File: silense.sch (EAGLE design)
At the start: 222 parts, among them IC1 AD8334ACPZ, IC3 LT8471EFE#PBF, J1 FMC-LPC

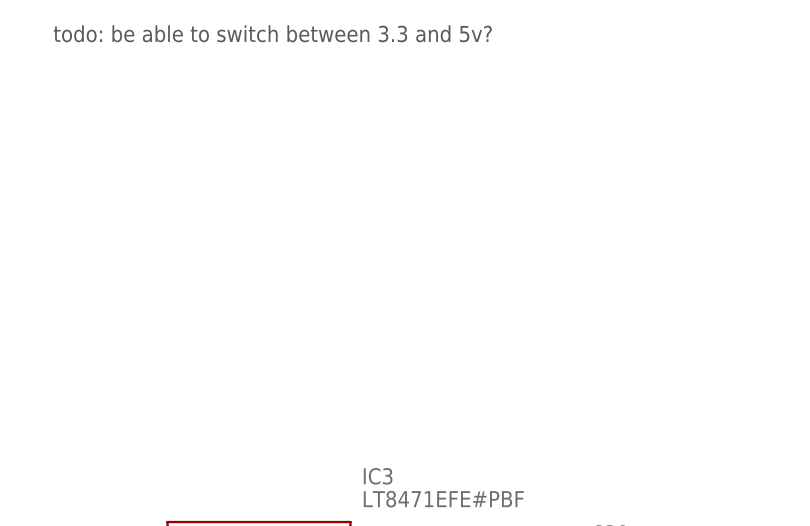
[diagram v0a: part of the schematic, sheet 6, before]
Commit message: added todos
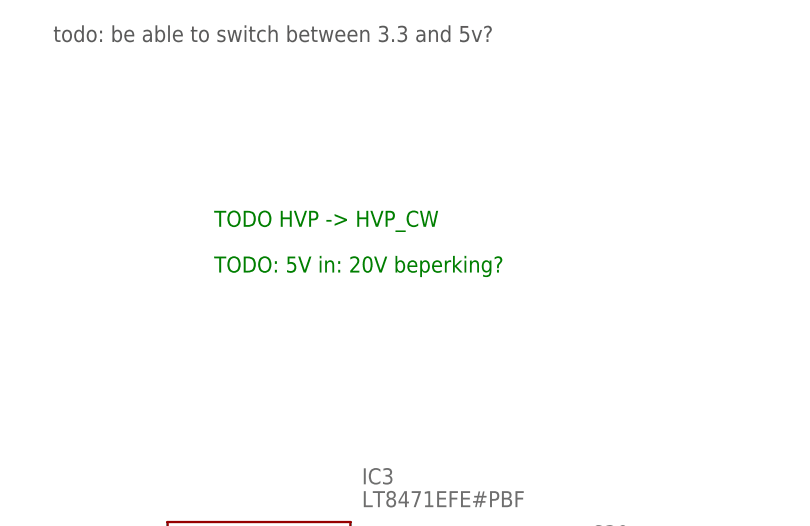
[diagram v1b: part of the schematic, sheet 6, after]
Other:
- note added: "TODO HVP -> HVP_CW"
- note added: "TODO: 5V in: 20V beperking?"
- note added: "TODO: Power supplies"
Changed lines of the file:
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@@
 <?xml version="1.0" encoding="utf-8"?>
 <!DOCTYPE eagle SYSTEM "eagle.dtd">
-<eagle version="9.5.1">
+<eagle version="9.5.0">
 <drawing>
 <settings>
@@
 <setting verticaltext="up"/>
 </settings>
-<grid distance="1" unitdist="mm" unit="mm" style="lines" multiple="1" display="yes" altdistance="0.5" altunitdist="mm" altunit="mm"/>
+<grid distance="0.1" unitdist="inch" unit="inch" style="lines" multiple="1" display="no" altdistance="0.01" altunitdist="inch" altunit="inch"/>
 <layers>
 <layer number="1" name="Top" color="4" fill="1" visible="no" active="no"/>
@@
 <text x="96.52" y="180.34" size="1.778" layer="91">TODO change impedance matching values</text>
 <text x="96.52" y="175.26" size="1.778" layer="91">TODO make ground symbols the same</text>
+<text x="147.32" y="223.52" size="1.778" layer="91">TODO: Power supplies</text>
 </plain>
 <instances>
@@
 <text x="38" y="18" size="1.778" layer="97">5V deduction</text>
 <text x="60.86" y="127.22" size="1.778" layer="97">todo: be able to switch between 3.3 and 5v?</text>
+<text x="78.74" y="106.68" size="1.778" layer="91">TODO HVP -&gt; HVP_CW</text>
+<text x="78.74" y="101.6" size="1.778" layer="91">TODO: 5V in: 20V beperking?</text>
 </plain>
 <instances>
